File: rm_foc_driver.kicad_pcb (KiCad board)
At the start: 4 copper layers, 70 x 70 mm, 78 parts, among them J1 SWD, J2 TMC4671, J3 UART, J4 TMC4671, J6 Conn_01x02, J8 Conn_01x03, Q1 CSD18540Q5B, Q2 CSD18540Q5B, Q3 CSD18540Q5B, Q4 CSD18540Q5B, Q5 CSD18540Q5B, Q6 CSD18540Q5B, U1 TPS54540, U10 74HC244, U2 RT9013, U3 STM32F401CCUx, U4 AMS1117-5.0, U5 IR2104, U6 INA2180, U7 MT6701, U8 IR2104, U9 IR2104, Y1 Crystal_GND24

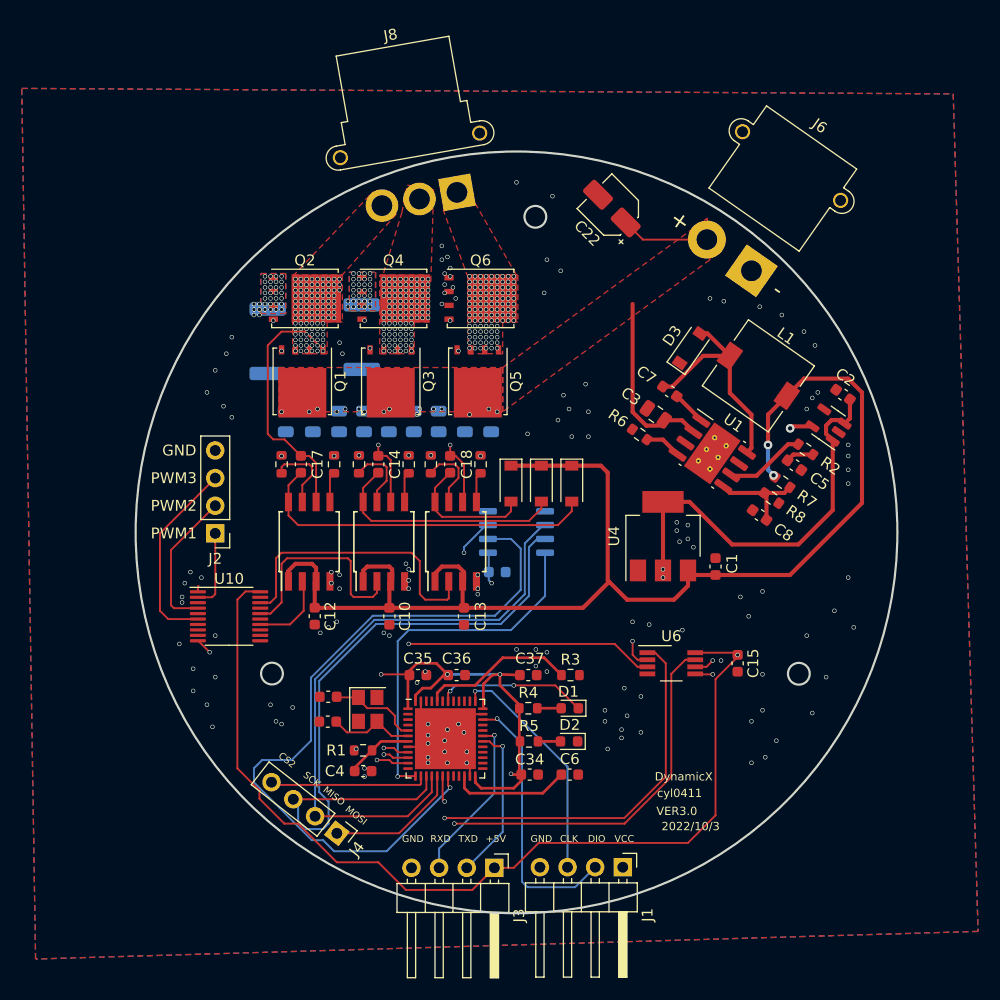
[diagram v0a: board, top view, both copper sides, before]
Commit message: correct some bug yesterday
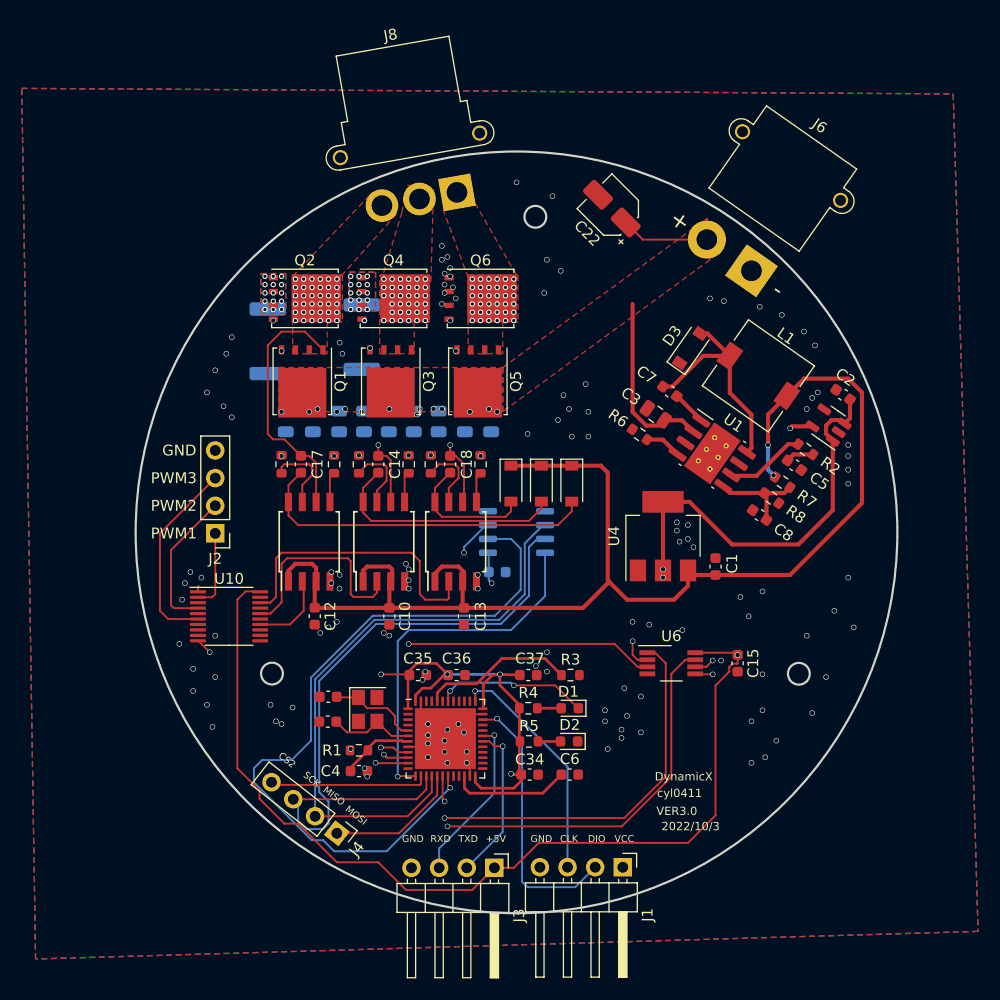
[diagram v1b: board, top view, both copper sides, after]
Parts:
- moved C4 0.38 mm to (150.6, 122.9)
- moved R1 0.38 mm to (150.6, 121.0)
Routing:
- net +3.3V: track 114.8 -> 116.6 mm
- net /SL_A: track 65.5 -> 66.8 mm, vias 35 -> 16
- net Net-(C4-Pad1): track 6.21 -> 6.75 mm
- net /SL_B: track 55.3 -> 55.2 mm, vias 31 -> 16
- net GND: vias 134 -> 129
- net /SH_C: vias 112 -> 37
- net /SH_B: vias 107 -> 35
- net /SH_A: vias 103 -> 36
- net +24V: vias 16 -> 14
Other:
- board text added: "Q2"
